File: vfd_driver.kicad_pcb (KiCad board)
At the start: 2 copper layers, 89.5 x 45.3 mm, 30 parts, among them J1 Input, J2 futaba_7_lt_44z, J3 High Volt, J4 FIL_n, J5 FIL_p, Q3 BC817, Q4 BC807, Q5 BC817, Q6 BC807, U1 74HC595, U2 74HC595, U3 74HC595, U4 74HC595, U5 TBD62783A, U6 TBD62783A, U7 TBD62783A

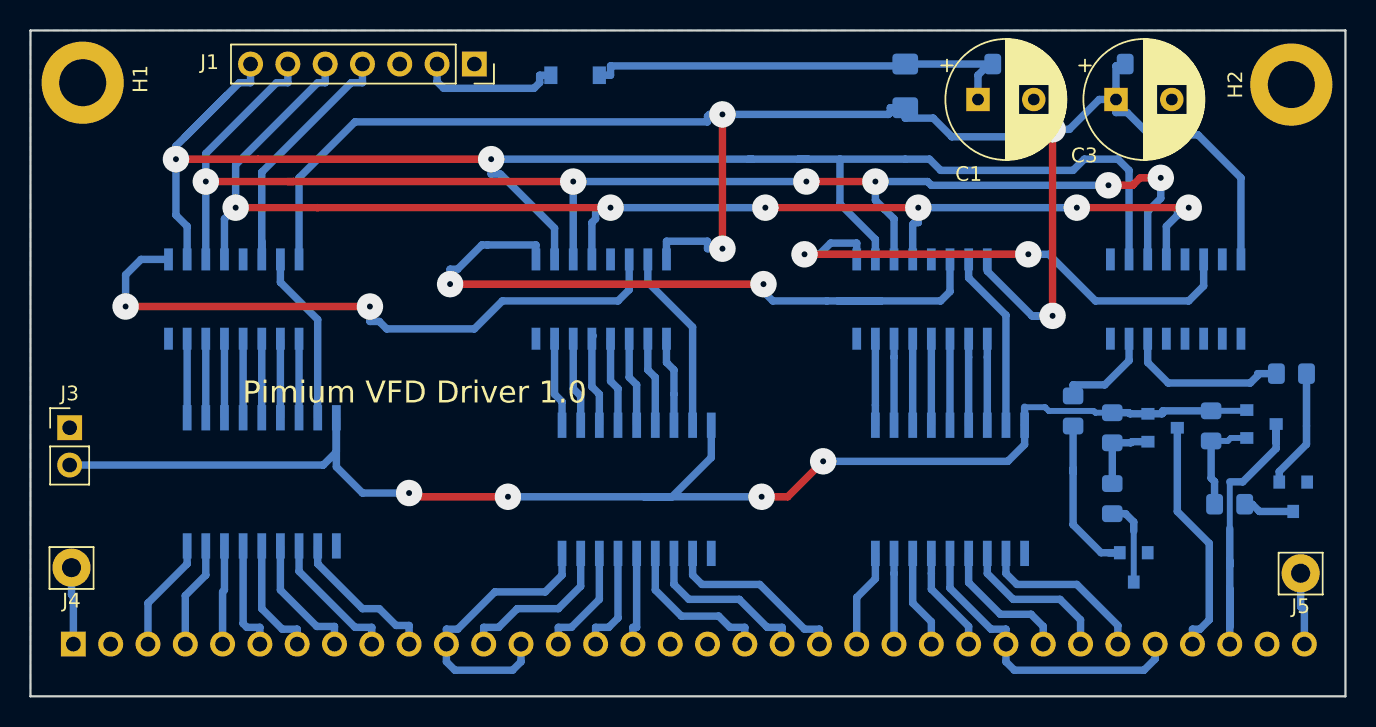
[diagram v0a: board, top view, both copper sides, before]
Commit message: arranging labels
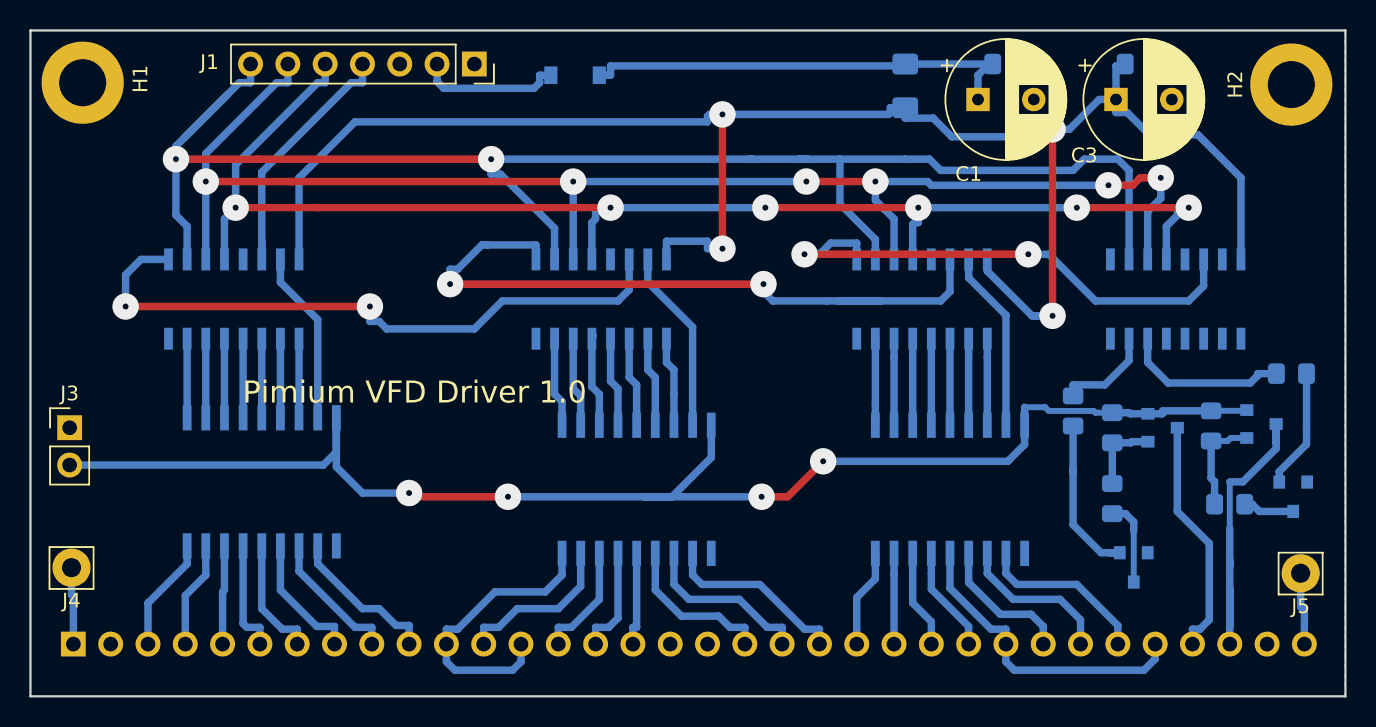
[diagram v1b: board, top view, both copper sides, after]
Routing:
- added copper zone on F.Cu, net GND
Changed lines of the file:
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@@
   (layers
     (0 F.Cu signal)
-    (31 B.Cu signal hide)
+    (31 B.Cu signal)
     (32 B.Adhes user)
     (33 F.Adhes user)
@@
   (segment (start 112.522 47.371) (end 113.538 46.355) (width 0.508) (layer B.Cu) (net 38))
   (segment (start 86.36 44.196) (end 101.219 44.196) (width 0.508) (layer F.Cu) (net 38))
-  (via (at 40.132 47.752) (size 1.8) (drill 0.4) (layers F.Cu B.Cu) (net 39))
+  (via (at 40.132 47.752) (size 1.8) (drill 0.4) (layers F.Cu B.Cu) (net 39) (status 1000000))
   (segment (start 41.816 44.544) (end 43.053 44.544) (width 0.4064) (layer B.Cu) (net 39) (status 20))
   (segment (start 40.132 47.752) (end 40.132 45.593) (width 0.508) (layer B.Cu) (net 39))
@@
       )
     )
+  )
+  (zone (net 1) (net_name GND) (layer F.Cu) (hatch edge 0.508)
+    (connect_pads (clearance 0.508))
+    (min_thickness 0.254)
+    (fill yes (arc_segments 16) (thermal_gap 0.508) (thermal_bridge_width 0.508))
+    (polygon
+      (pts
+        (xy 33.655 28.956) (xy 123.19 28.956) (xy 123.19 74.295) (xy 33.655 74.295)
+      )
+    )
